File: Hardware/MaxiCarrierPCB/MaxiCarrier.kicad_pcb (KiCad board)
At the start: 2 copper layers, 75.5 x 37.2 mm, 1 part, among them J1 ET60T-D02-3-08-D02-X-R1-S

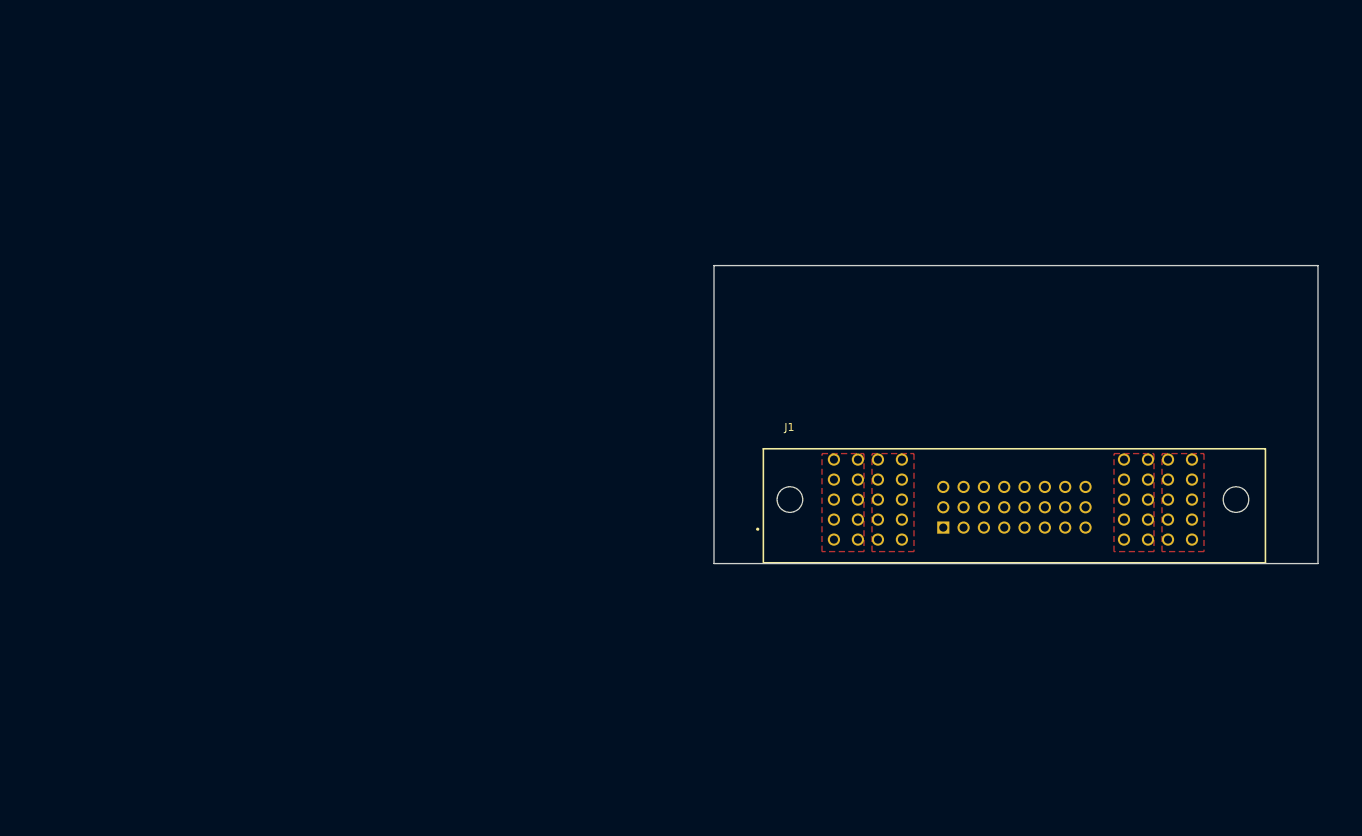
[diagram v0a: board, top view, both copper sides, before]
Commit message: more sch + some footprints
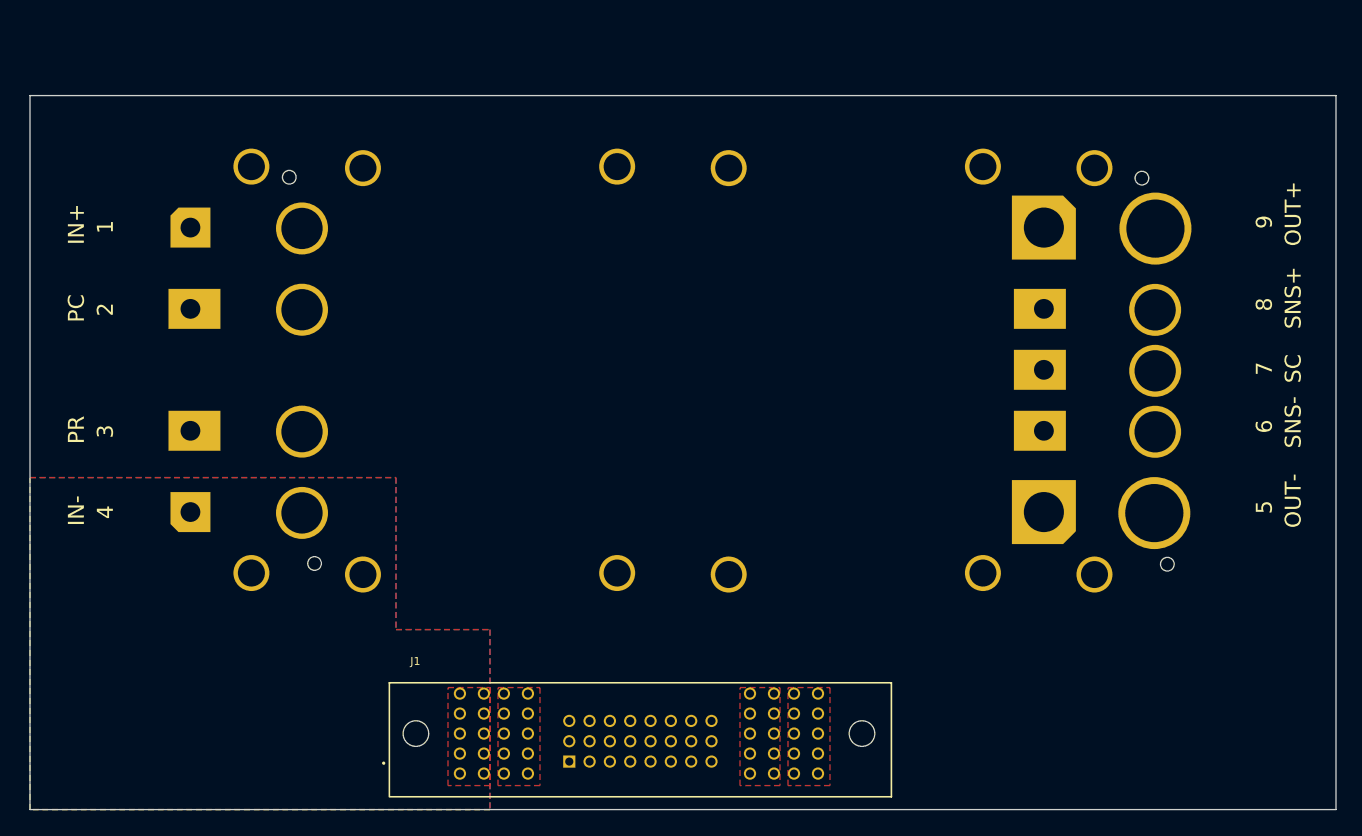
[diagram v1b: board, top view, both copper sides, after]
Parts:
- added U1: ~, UTSVT_Connectors:Vicor_Maxi_Brick, F.Cu at (31.3, 103.1)
- moved J1 55.1 mm to (97.0, 114.8)
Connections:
- J1 pad 01: unconnected-(J1-Pad01) -> /PC
- J1 pad 03: unconnected-(J1-Pad03) -> /SC
- J1 pad 05: unconnected-(J1-Pad05) -> /SNS+
- J1 pad 07: unconnected-(J1-Pad07) -> /SNS-
- J1 pad P01: IN+ -> IN-
- J1 pad P02: IN- -> Unfused_IN+
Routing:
- added copper zone on B.Cu, net IN-
- added copper zone on F.Cu, net Unfused_IN+
- removed copper zone on F.Cu, net IN+
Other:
- board size 75.5 x 37.2 mm -> 163.2 x 89.2 mm

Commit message: holy fatass
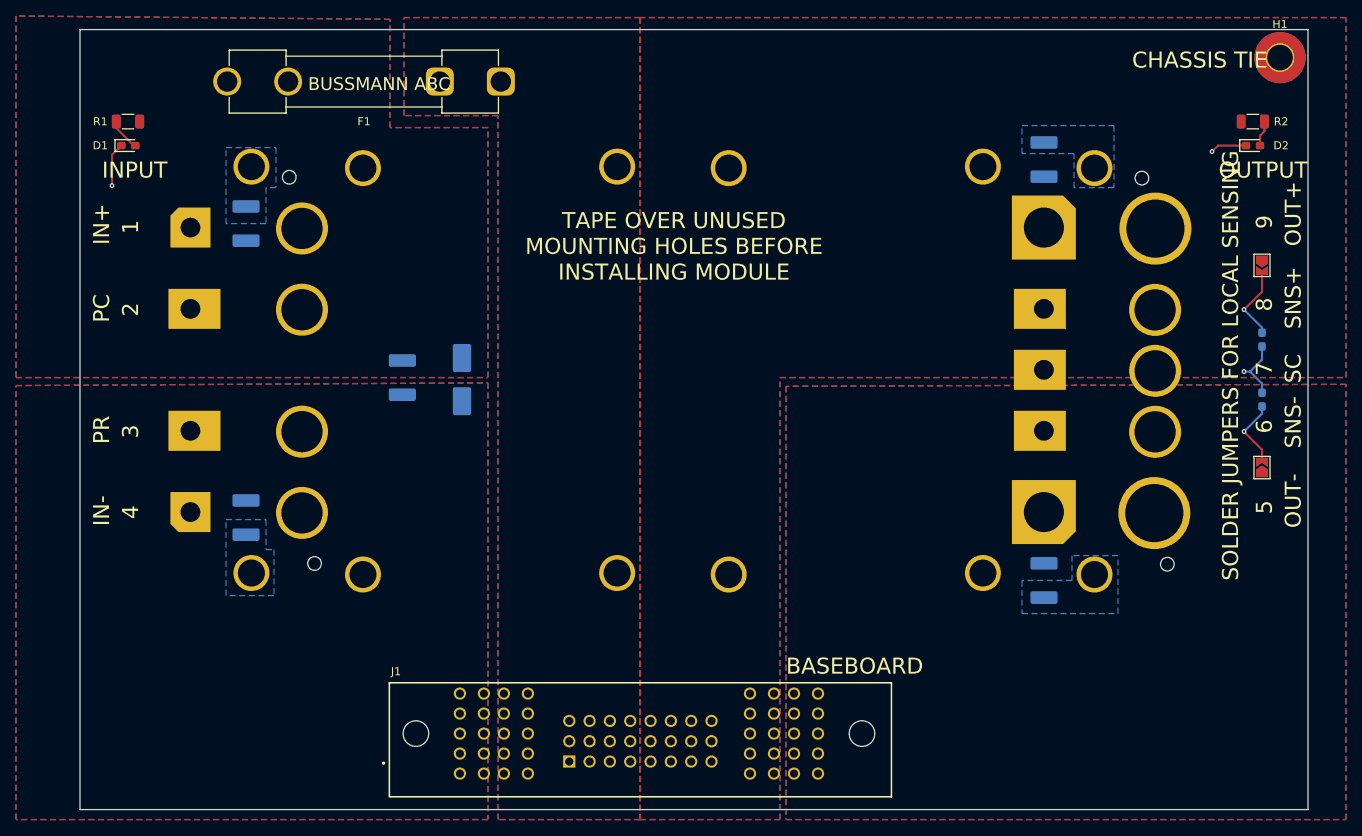
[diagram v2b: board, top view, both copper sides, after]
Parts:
- added C1: 0.2uF, Capacitor_SMD:C_1812_4532Metric_Pad1.57x3.40mm_HandSolder, B.Cu at (67.3, 70.2)
- added C2: 4.7nF, Capacitor_SMD:C_1812_4532Metric_Pad1.57x3.40mm_HandSolder, B.Cu at (47.8, 51.0)
- added C3: 4.7nF, Capacitor_SMD:C_1812_4532Metric_Pad1.57x3.40mm_HandSolder, B.Cu at (47.8, 87.8)
- added C4: 4.7nF, Capacitor_SMD:C_1812_4532Metric_Pad1.57x3.40mm_HandSolder, B.Cu at (147.5, 43.0)
- added C5: 4.7nF, Capacitor_SMD:C_1812_4532Metric_Pad1.57x3.40mm_HandSolder, B.Cu at (147.5, 95.6)
- added D1: LED, LED_SMD:LED_0603_1608Metric_Pad1.05x0.95mm_HandSolder, F.Cu at (33.0, 41.2)
- added D2: LED, LED_SMD:LED_0603_1608Metric_Pad1.05x0.95mm_HandSolder, F.Cu at (173.6, 41.2)
- added D3: TVS, Diode_SMD:D_SMB_Handsoldering, B.Cu at (74.8, 70.5)
- added F1: Fuse, Fuse:Fuseholder_Clip-6.3x32mm_Littelfuse_122_Inline_P34.21x7.62mm_D2.54mm_Horizontal, F.Cu at (79.6, 33.2)
- added H1: MountingHole_Pad, MountingHole:MountingHole_3.2mm_M3_Pad_TopBottom, F.Cu at (177.0, 30.2)
- added JP1: SNS+, Jumper:SolderJumper-2_P1.3mm_Open_TrianglePad1.0x1.5mm, F.Cu at (174.8, 56.2)
- added JP2: SNS-, Jumper:SolderJumper-2_P1.3mm_Open_TrianglePad1.0x1.5mm, F.Cu at (174.8, 81.5)
- added LOGO1: Dr. Hallock, UTSVT_Logos:Hallock_Image, B.Cu at (101.8, 69.5)
- added LOGO2: LHRs, UTSVT_Logos:LHRs_LOGO, F.Cu at (35.2, 118.5)
- added R1: R, Resistor_SMD:R_1206_3216Metric, F.Cu at (33.0, 38.2)
- added R2: R, Resistor_SMD:R_1206_3216Metric, F.Cu at (173.6, 38.2)
- added R3: Ru, Capacitor_SMD:C_0603_1608Metric_Pad1.08x0.95mm_HandSolder, B.Cu at (174.8, 65.5)
- added R4: Rd, Capacitor_SMD:C_0603_1608Metric_Pad1.08x0.95mm_HandSolder, B.Cu at (174.8, 73.0)
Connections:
- J1 pad 03: /SC -> /SNS+
- J1 pad 05: /SNS+ -> /SC
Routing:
- net /SNS+: track 0.00 -> 120.3 mm, vias 0 -> 1
- net /SC: track 0.00 -> 107.3 mm, vias 0 -> 1
- net /SNS-: track 0.00 -> 103.8 mm, vias 0 -> 1
- net /PC: track 0.00 -> 85.0 mm
- net OUT-: track 0.00 -> 76.1 mm, vias 0 -> 1
- net IN-: track 0.00 -> 50.4 mm, vias 0 -> 1
- net Net-(D1-A): track 0.00 -> 4.08 mm
- net Net-(D2-A): track 0.00 -> 3.23 mm
- added copper zone on B.Cu, net IN+
- added copper zone on F.Cu, net IN+
- added copper zone on B.Cu, net OUT+
- added copper zone on B.Cu, net OUT-
- added copper zone on B.Cu, net PLATE
- added copper zone on In1.Cu, net PLATE
- added copper zone on In2.Cu, net PLATE
- added copper zone on B.Cu, net Unfused_IN+
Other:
- board size 163.2 x 89.2 mm -> 153.5 x 97.5 mm
- copper layers 2 -> 4
- board text added: "BASEBOARD"
- board text added: "BUSSMANN ABC"
- board text added: "CHASSIS TIE"
- board text added: "DOWN"
- board text added: "INPUT"
- board text added: "Maxi DC-DC Carrier Ravi Shah 2025"
- board text added: "NC FOR NOMINAL OUTPUT VOLTAGE"
- board text added: "OUTPUT"
- board text added: "SOLDER JUMPERS FOR LOCAL SENSING"
- board text added: "TAPE OVER UNUSED MOUNTING HOLES BEFORE INSTALLING MODULE"
- board text added: "TRIM"
- board text added: "UP"
- board text added: "draw funny lines warnings shrink as much as possible"
